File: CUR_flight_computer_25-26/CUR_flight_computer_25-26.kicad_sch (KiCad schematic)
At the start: 0 parts

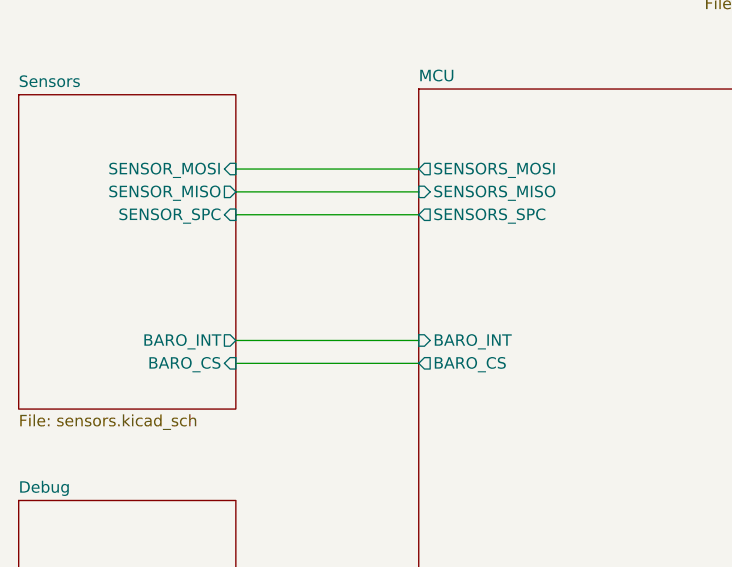
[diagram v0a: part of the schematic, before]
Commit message: Magnitomer
Put In Magnitominer
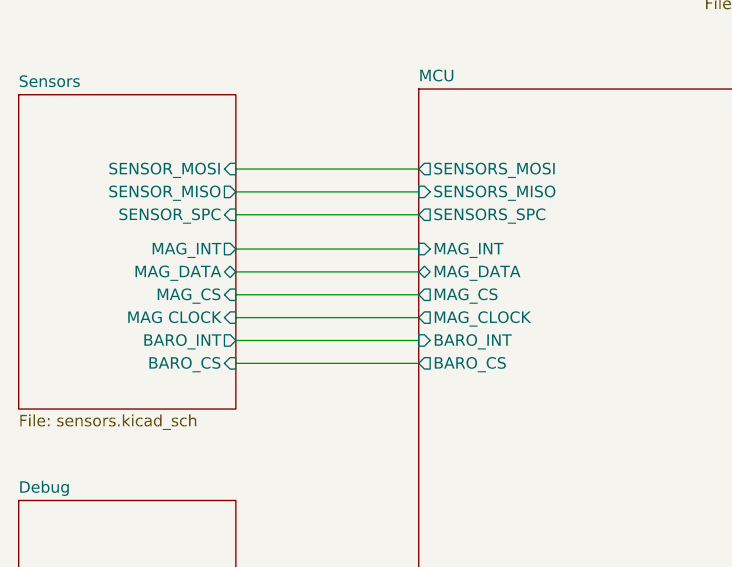
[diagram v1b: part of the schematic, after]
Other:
- sheet MCU ports: added MAG_CLOCK, MAG_CS, MAG_DATA, MAG_INT; removed none
- sheet Sensors ports: added MAG CLOCK, MAG_CS, MAG_DATA, MAG_INT; removed none
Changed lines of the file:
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@@
+	(wire
+		(pts
+			(xy 93.98 77.47) (xy 114.3 77.47)
+		)
+		(stroke
+			(width 0)
+			(type default)
+		)
+	)
+	(wire
+		(pts
+			(xy 93.98 69.85) (xy 114.3 69.85)
+		)
+		(stroke
+			(width 0)
+			(type default)
+		)
+	)
 	(wire
 		(pts
@@
 		(pts
 			(xy 93.98 60.96) (xy 114.3 60.96)
+		)
+		(stroke
+			(width 0)
+			(type default)
+		)
+	)
+	(wire
+		(pts
+			(xy 93.98 74.93) (xy 114.3 74.93)
+		)
+		(stroke
+			(width 0)
+			(type default)
+		)
+	)
+	(wire
+		(pts
+			(xy 93.98 72.39) (xy 114.3 72.39)
 		)
 		(stroke
@@
 			)
 		)
+		(pin "MAG_CLOCK" output
+			(at 114.3 77.47 180)
+			(effects
+				(font
+					(size 1.27 1.27)
+				)
+				(justify left)
+			)
+		)
+		(pin "MAG_CS" output
+			(at 114.3 74.93 180)
+			(effects
+				(font
+					(size 1.27 1.27)
+				)
+				(justify left)
+			)
+		)
+		(pin "MAG_DATA" bidirectional
+			(at 114.3 72.39 180)
+			(effects
+				(font
+					(size 1.27 1.27)
+				)
+				(justify left)
+			)
+		)
+		(pin "MAG_INT" input
+			(at 114.3 69.85 180)
+			(effects
+				(font
+					(size 1.27 1.27)
+				)
+				(justify left)
+			)
+		)
 		(instances
 			(project "CUR_flight_computer_25-26"
@@
 			(effects
 				(font
+					(size 1.27 1.27)
+				)
+				(justify right)
+			)
+		)
+		(pin "MAG CLOCK" input
+			(at 93.98 77.47 0)
+			(effects
+				(font
+					(size 1.27 1.27)
+				)
+				(justify right)
+			)
+		)
+		(pin "MAG_CS" input
+			(at 93.98 74.93 0)
+			(effects
+				(font
+					(size 1.27 1.27)
+				)
+				(justify right)
+			)
+		)
+		(pin "MAG_DATA" bidirectional
+			(at 93.98 72.39 0)
+			(effects
+				(font
+					(size 1.27 1.27)
+				)
+				(justify right)
+			)
+		)
+		(pin "MAG_INT" output
+			(at 93.98 69.85 0)
+			(effects
+				(font
